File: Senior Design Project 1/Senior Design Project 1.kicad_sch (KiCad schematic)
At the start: 29 parts, among them U1 74LS05, U2 74HC273, U3 LM393NG, U6 LM555xN, U9 74HC273

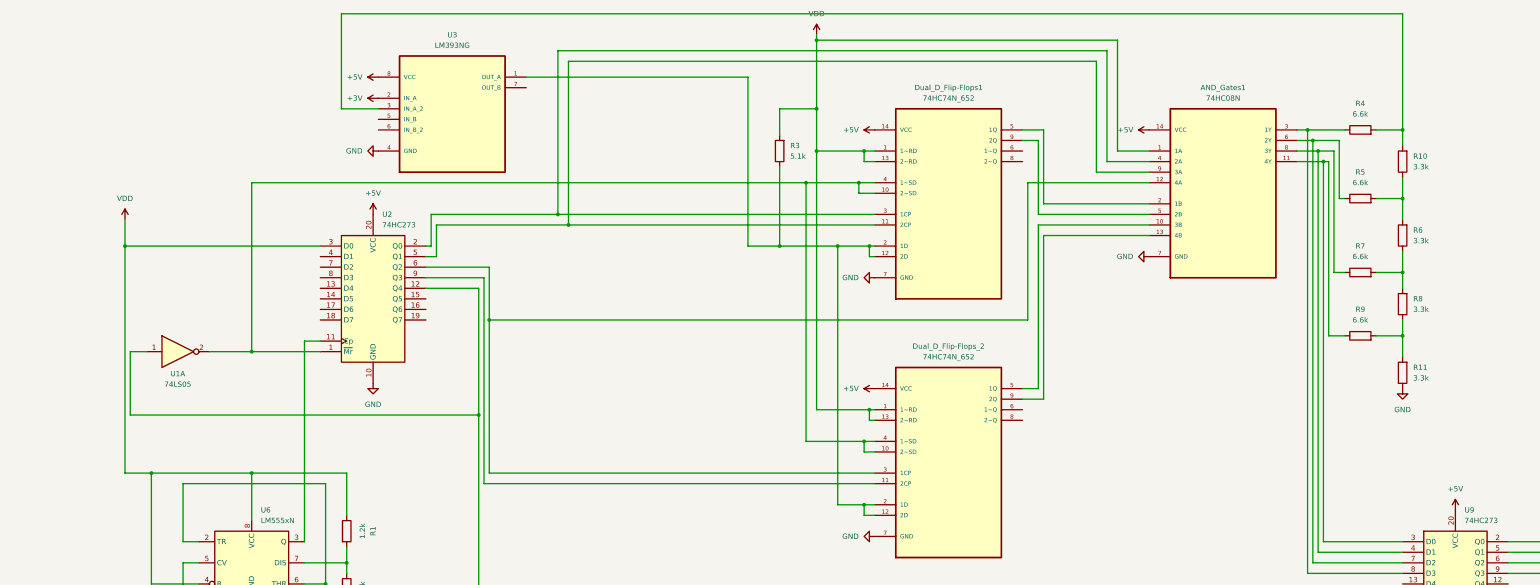
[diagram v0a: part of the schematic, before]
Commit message: Updated Schematic & PCB
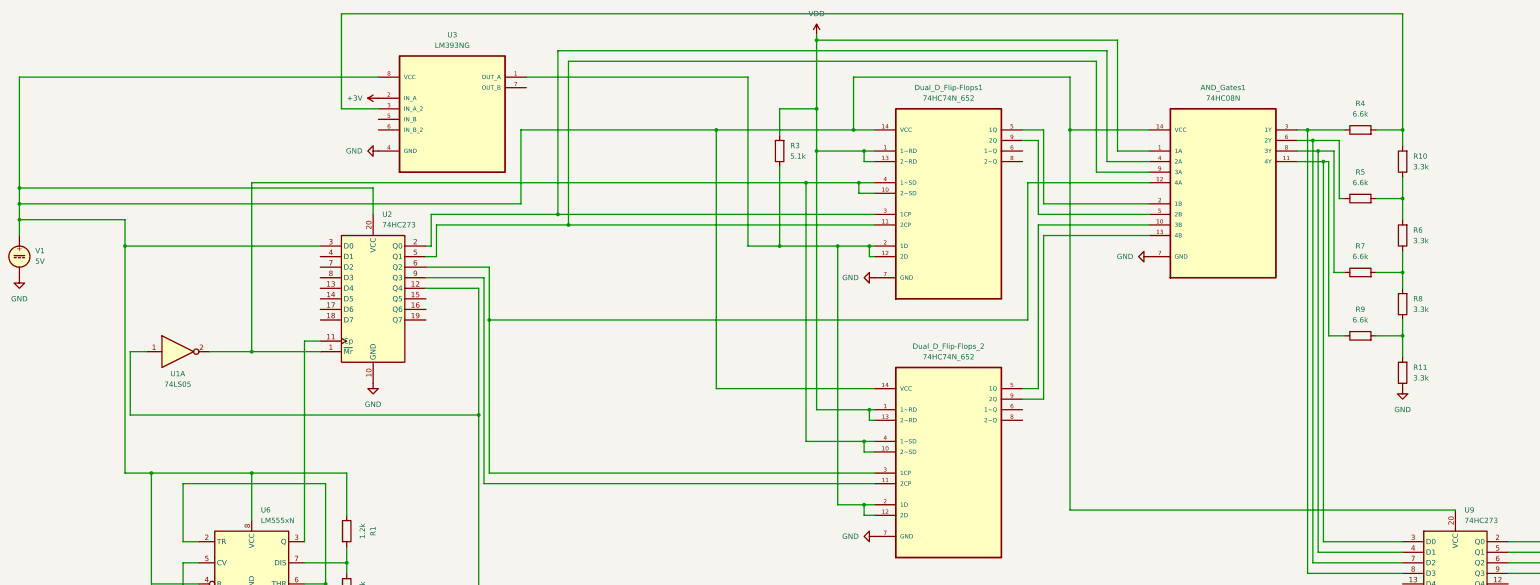
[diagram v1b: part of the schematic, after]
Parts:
- added V1: 5V, TerminalBlock:TerminalBlock_bornier-3_P5.08mm, symbol Simulation_SPICE:VDC
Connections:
- net GND: now also V1.2
- net VDD: no longer R1.1, U2.3 (D0), U6.4 (R), U6.8 (VCC)
- net +5V: no longer names the net of AND_Gates1.14 (VCC), Dual_D_Flip-Flops1.14 (VCC), Dual_D_Flip-Flops_2.14 (VCC), U2.20 (VCC), U3.8 (VCC), U9.20 (VCC)
- net +5V: now also R1.1, U2.3 (D0), U6.4 (R), U6.8 (VCC), V1.1
